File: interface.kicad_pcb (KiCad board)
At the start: 2 copper layers, 36.8 x 66 mm, 35 parts, among them U1 THERMAL, U2 SX1308

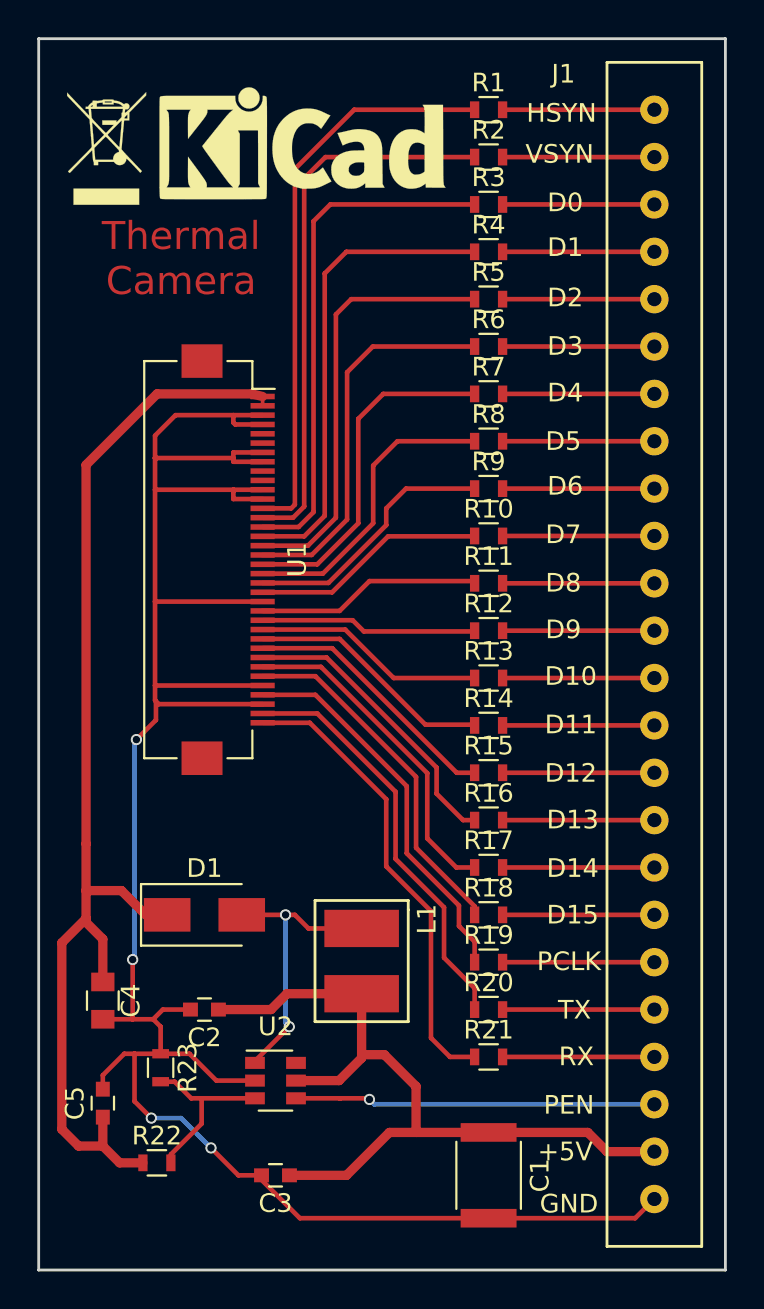
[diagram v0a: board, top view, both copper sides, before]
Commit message: finish and factory
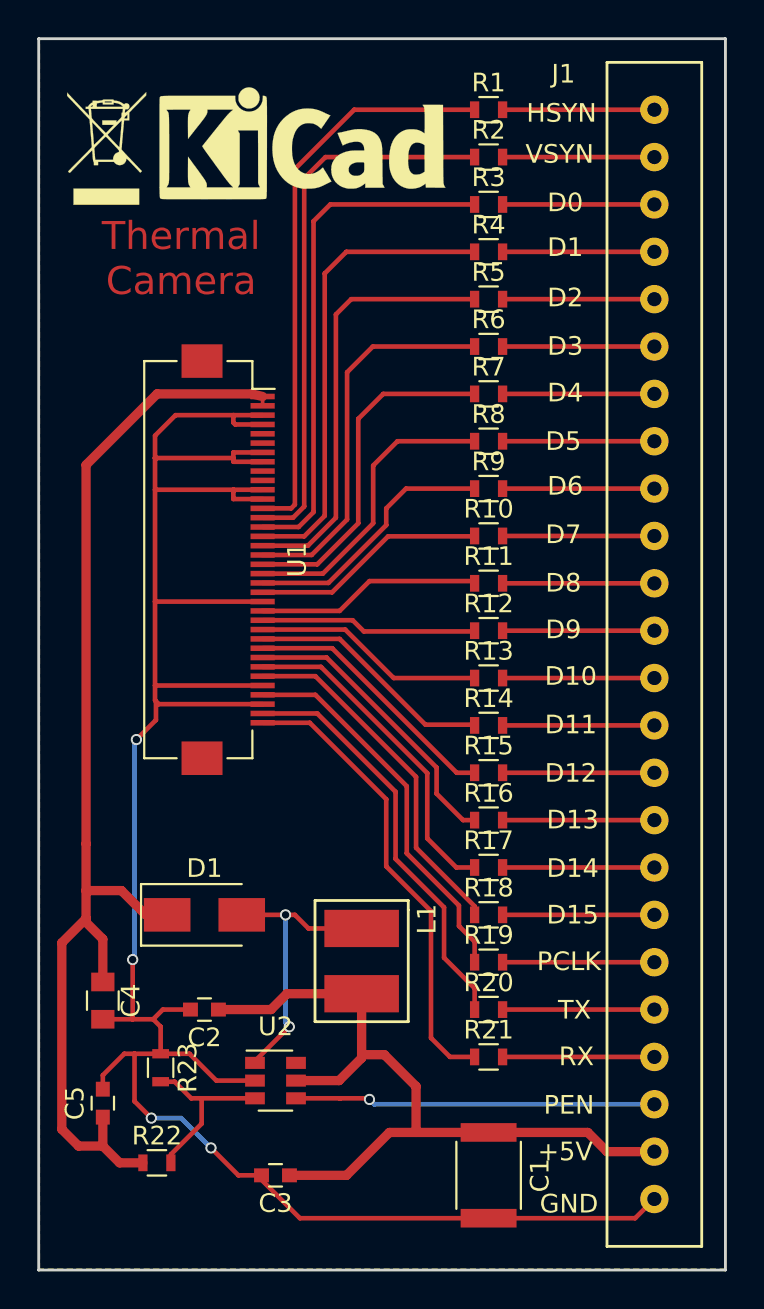
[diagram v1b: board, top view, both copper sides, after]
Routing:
- added copper zone on B.Cu, net GND
- added copper zone on F.Cu, net GND
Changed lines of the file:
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@@
     (trace_clearance 0.15)
     (zone_clearance 0.508)
-    (zone_45_only no)
+    (zone_45_only yes)
     (trace_min 0.2)
     (segment_width 0.2)
@@
   (segment (start 141.6 80.6) (end 141.6 75) (width 0.25) (layer F.Cu) (net 52))
   (segment (start 139.4 82.8) (end 141.6 80.6) (width 0.25) (layer F.Cu) (net 52))
+  (zone (net 0) (net_name "") (layer F.Cu) (hatch edge 0.508)
+    (connect_pads (clearance 0.508))
+    (min_thickness 0.254)
+    (keepout (tracks allowed) (vias allowed) (copperpour not_allowed))
+    (fill (arc_segments 16) (thermal_gap 0.508) (thermal_bridge_width 0.508))
+    (polygon
+      (pts
+        (xy 143.9 104.8) (xy 139.5 104.8) (xy 139.5 103.4) (xy 143.9 103.4)
+      )
+    )
+  )
+  (zone (net 0) (net_name "") (layer F.Cu) (hatch edge 0.508)
+    (connect_pads (clearance 0.508))
+    (min_thickness 0.254)
+    (keepout (tracks allowed) (vias allowed) (copperpour not_allowed))
+    (fill (arc_segments 16) (thermal_gap 0.508) (thermal_bridge_width 0.508))
+    (polygon
+      (pts
+        (xy 147 113.8) (xy 150.2 113.8) (xy 150.2 117.3) (xy 146.9 117.3) (xy 146.9 113.8)
+      )
+    )
+  )
+  (zone (net 0) (net_name "") (layer F.Cu) (hatch edge 0.508)
+    (connect_pads (clearance 0.508))
+    (min_thickness 0.254)
+    (keepout (tracks allowed) (vias allowed) (copperpour not_allowed))
+    (fill (arc_segments 16) (thermal_gap 0.508) (thermal_bridge_width 0.508))
+    (polygon
+      (pts
+        (xy 130.4 73.7) (xy 131.2 74.5) (xy 127.8 77.9) (xy 127.8 99.2) (xy 131.2 99.2)
+        (xy 131.2 103.1) (xy 129.1 103.1) (xy 129.1 102.9) (xy 127.8 100.368421) (xy 127.8 102.2)
+        (xy 128.3 102.2) (xy 129 102.9) (xy 129 110.9) (xy 130.2 112.1) (xy 130.2 114.8)
+        (xy 128.6 114.8) (xy 127.9 114.1) (xy 126.6 114.1) (xy 125.7 113.2) (xy 125.7 103.2)
+        (xy 126.6 102.3) (xy 126.4 102.3) (xy 126.4 77.2) (xy 130.2 73.4) (xy 130.4 73.4)
+      )
+    )
+  )
+  (zone (net 0) (net_name "") (layer F.Cu) (hatch edge 0.508)
+    (connect_pads (clearance 0.508))
+    (min_thickness 0.254)
+    (keepout (tracks allowed) (vias allowed) (copperpour not_allowed))
+    (fill (arc_segments 16) (thermal_gap 0.508) (thermal_bridge_width 0.508))
+    (polygon
+      (pts
+        (xy 134.5 103.1) (xy 132.3 103.1) (xy 132.3 99.9) (xy 134.5 99.9)
+      )
+    )
+  )
+  (zone (net 2) (net_name GND) (layer F.Cu) (hatch edge 0.508)
+    (connect_pads (clearance 0.508))
+    (min_thickness 0.254)
+    (fill yes (arc_segments 16) (thermal_gap 0.508) (thermal_bridge_width 0.508))
+    (polygon
+      (pts
+        (xy 161.3 120.6) (xy 124.5 120.6) (xy 124.5 54.6) (xy 161.3 54.6)
+      )
+    )
+  )
+  (zone (net 2) (net_name GND) (layer B.Cu) (hatch edge 0.508)
+    (connect_pads (clearance 0.508))
+    (min_thickness 0.254)
+    (fill yes (arc_segments 16) (thermal_gap 0.508) (thermal_bridge_width 0.508))
+    (polygon
+      (pts
+        (xy 161.3 120.6) (xy 124.5 120.6) (xy 124.5 54.6) (xy 161.3 54.6)
+      )
+    )
+  )
 )
